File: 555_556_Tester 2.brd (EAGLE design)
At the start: 40.6 x 38.1 mm, 19 parts, among them IC1 556, J2 POWER_JACKPTH

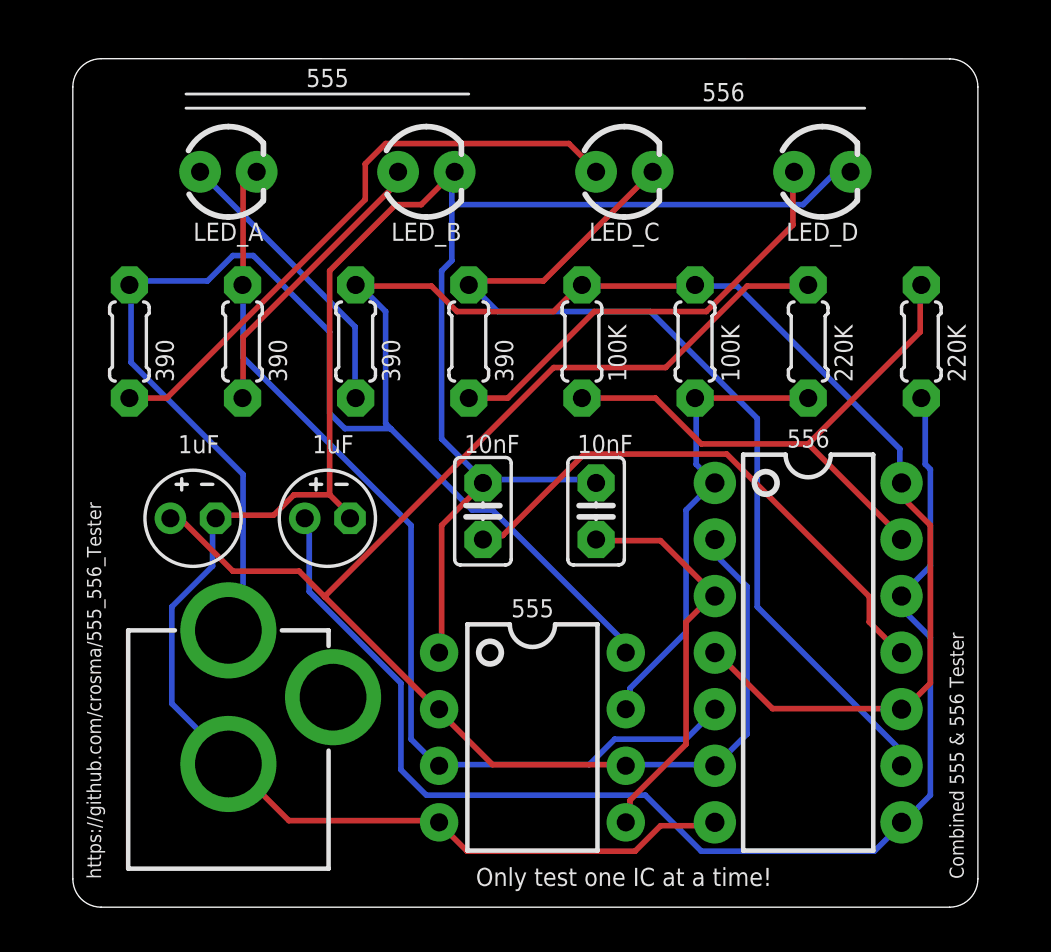
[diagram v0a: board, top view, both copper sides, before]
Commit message: Revisions
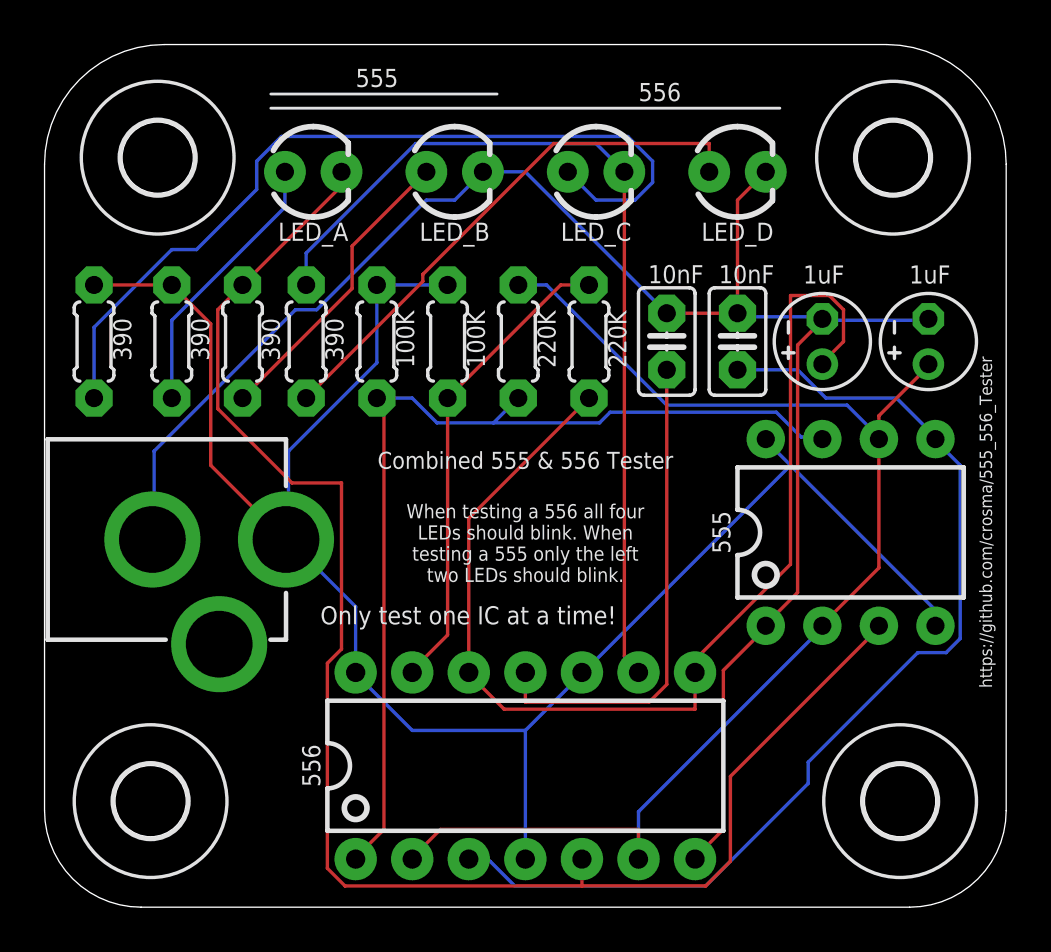
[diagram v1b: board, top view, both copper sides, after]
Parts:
- added U$1, U$2, U$3, U$4: (no value), holes:3,2
- moved C1 34.0 mm to (39.7, 25.4), turned to 90 degrees
- moved C2 23.6 mm to (34.9, 25.4), turned to 90 degrees
- moved J2 21.0 mm to (-2.86, 16.5), turned to 270 degrees
- moved 555 17.0 mm to (36.2, 16.8), turned to 0 degrees
- moved R7 14.9 mm to (24.4, 25.4)
- moved R5 14.3 mm to (14.9, 25.4)
- moved R8 13.0 mm to (21.3, 25.4)
- moved IC1 12.0 mm to (22.9, 6.35), turned to 0 degrees
- moved C4 11.2 mm to (27.9, 25.4)
- moved C3 9.92 mm to (31.1, 25.4)
- moved R1 8.26 mm to (5.71, 25.4)
- moved R3 7.30 mm to (11.7, 25.4)
- moved R6 6.03 mm to (18.1, 25.4)
- moved D1 3.81 mm to (12.1, 33.0)
- moved D3 3.81 mm to (31.1, 33.0)
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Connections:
- net +5V: now also 555.4
- net GND: no longer 555.4
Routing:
- net CV: track 18.3 -> 47.4 mm
- net GND: track 108.6 -> 80.4 mm
- net OUT: track 44.1 -> 70.9 mm
- net +5V: track 108.6 -> 83.6 mm
- net DIS: track 21.2 -> 44.1 mm
- net N$8: track 27.2 -> 38.6 mm
- net THR_TRIG: track 68.0 -> 58.8 mm
- net THR2_TRIG2: track 58.7 -> 51.3 mm
- net DIS2: track 26.3 -> 21.4 mm
- net N$6: track 20.2 -> 24.3 mm
- net OUT2: track 44.1 -> 41.0 mm
- net CV2: track 24.7 -> 22.1 mm
- net N$1: track 13.1 -> 12.3 mm
- net N$2: track 13.1 -> 13.6 mm
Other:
- board size 40.6 x 38.1 mm -> 43.2 x 38.7 mm
- board text added: "When testing a 556 all four LEDs should blink. When testing a 555 only the left two LEDs should blink."
